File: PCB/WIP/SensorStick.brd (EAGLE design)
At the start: 58.4 x 69.5 mm, 89 parts, among them U1 TPD4F003DQDR, U10 LIS3MDLTR, U11 LIS3MDLTR, U2 BMI088, U3 BMI088, U4 BMI088, U5 STM32H743ZIT6, U9 LIS3MDLTR, Y1 ECS-TXO-3225MV-400-TR

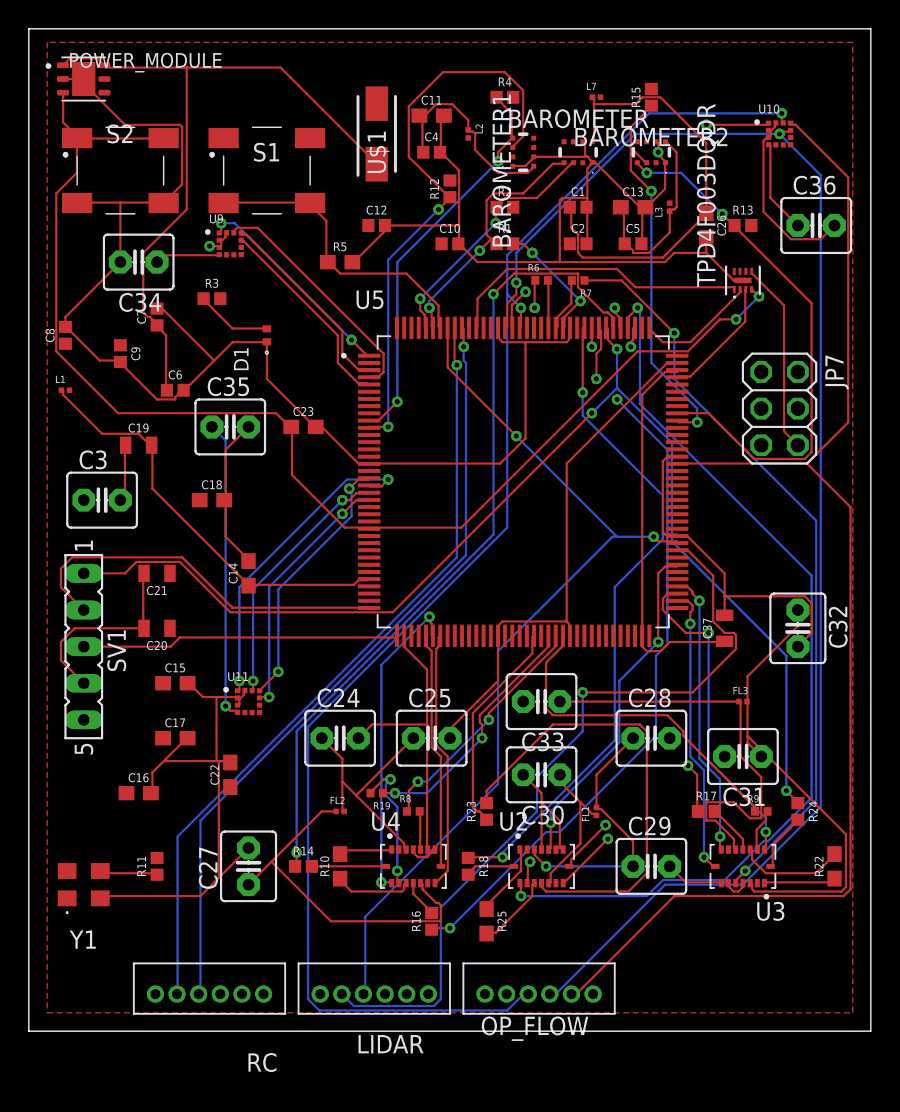
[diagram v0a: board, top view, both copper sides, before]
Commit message: first draft pretty much
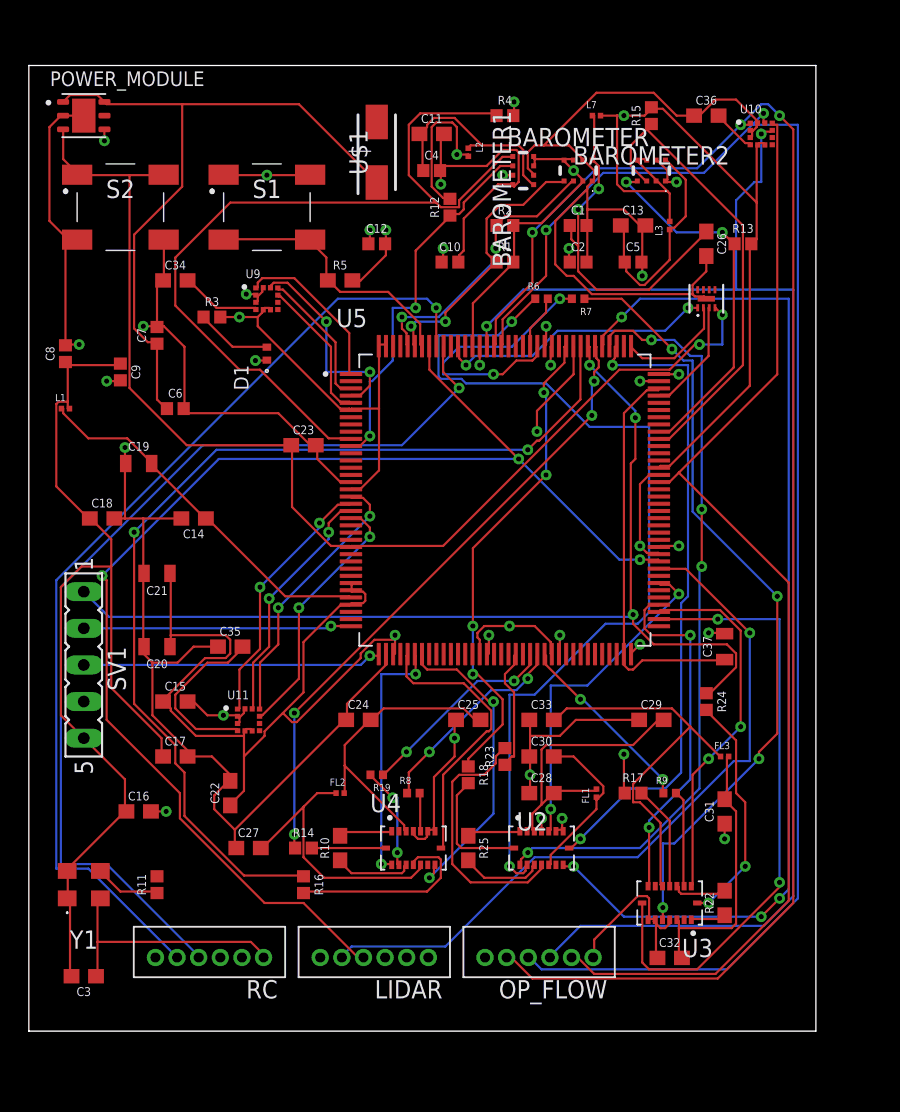
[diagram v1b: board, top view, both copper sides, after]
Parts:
- removed JP7: (no value), pinhead:2X03
- C24, C25, C27, C28, C29, C30, C31, C32, C33: value 0.1uf -> 0.1uF; device capacitor-wima:C2.5-4 -> SparkFun-Capacitors:0603
- C3, C34, C35, C36: device capacitor-wima:C2.5-4 -> SparkFun-Capacitors:0603
- moved C3 33.0 mm to (3.81, 3.81), turned to 180 degrees
- moved C32 24.5 mm to (44.5, 5.08), turned to 0 degrees
- moved C35 15.2 mm to (14.0, 26.7)
- moved C36 10.8 mm to (47.0, 63.5)
- moved C29 10.2 mm to (43.2, 21.6)
- moved R24 9.92 mm to (47.0, 22.9)
- moved R16 9.25 mm to (19.1, 10.2), turned to 270 degrees
- moved C28 8.52 mm to (35.6, 16.5)
- moved R22 8.03 mm to (48.3, 8.89)
- moved C18 7.73 mm to (5.08, 35.6)
- moved R9 6.48 mm to (44.5, 16.5)
- moved R18 6.35 mm to (30.5, 17.8)
- moved U3 5.68 mm to (44.5, 8.89)
- moved C14 5.39 mm to (11.4, 35.6), turned to 180 degrees
- moved R17 5.24 mm to (41.9, 16.5)
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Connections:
- removed net SWCLK_O1: JP7.3
- removed net SWDIO_O1: JP7.5
- removed net SWO_O1: JP7.1
- removed net USART1_RX: JP7.4
- removed net USART1_TX: JP7.2
- net 3V2: now also C28.2, C29.2; no longer C28.1, C29.1
- net 3V3: now also C3.2; no longer C3.1
- net 3V4: now also C24.2, C25.2; no longer C24.1, C25.1
- net 3V5: now also C31.2, C32.2; no longer C31.1, C32.1
- net GND: now also C24.1, C25.1, C27.1, C28.1, C29.1, C3.1, C30.1, C31.1, C32.1, C33.1, C34.1, C35.1, C36.1; no longer C24.2, C25.2, C27.2, C28.2, C29.2, C3.2, C30.2, C31.2, C32.2, C33.2, C34.2, C35.2, C36.2
- net N$10: now also C33.2; no longer C33.1
- net N$11: now also C36.2; no longer C36.1
- net N$4: now also C34.2; no longer C34.1
- net N$7: now also C35.2; no longer C35.1
- net N$8: now also C27.2; no longer C27.1
- net N$9: now also C30.2; no longer C30.1
- net NRST_O: no longer JP7.6
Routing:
- net 3V3: track 8.78 -> 263.0 mm, vias 2 -> 18
- net GND: track 348.3 -> 288.0 mm, vias 2 -> 23
- net SPI6_SCK: track 75.6 -> 108.6 mm, vias 2 -> 3
- net I2C2_SCL: track 27.5 -> 58.8 mm, vias 2 -> 0
- net SPI3_MOSI: track 44.9 -> 73.6 mm, vias 2 -> 4
- net I2C4_SDA: track 62.9 -> 91.2 mm, vias 2 -> 3
- net CSB_ACCEL3: track 42.2 -> 65.3 mm
- net SPI2_SCK: track 20.2 -> 43.2 mm
- net GPIO_EXTI2: track 52.1 -> 69.6 mm, vias 3 -> 2
- net N$14: track 3.79 -> 19.3 mm, vias 0 -> 2
- net UART5_RX: track 54.0 -> 68.2 mm
- net EXTI0_1: track 32.1 -> 18.1 mm
- net UART5_TX: track 54.3 -> 68.3 mm
- net I2C2_SDA: track 40.3 -> 26.3 mm
- net 3V5: track 32.5 -> 19.0 mm
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- added copper zone on layer 15, net 3V3
- removed copper zone on layer 1, net 3V3
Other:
- board size 58.4 x 69.5 mm -> 54.6 x 67 mm
